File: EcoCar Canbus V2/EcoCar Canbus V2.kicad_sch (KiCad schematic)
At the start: 7 parts

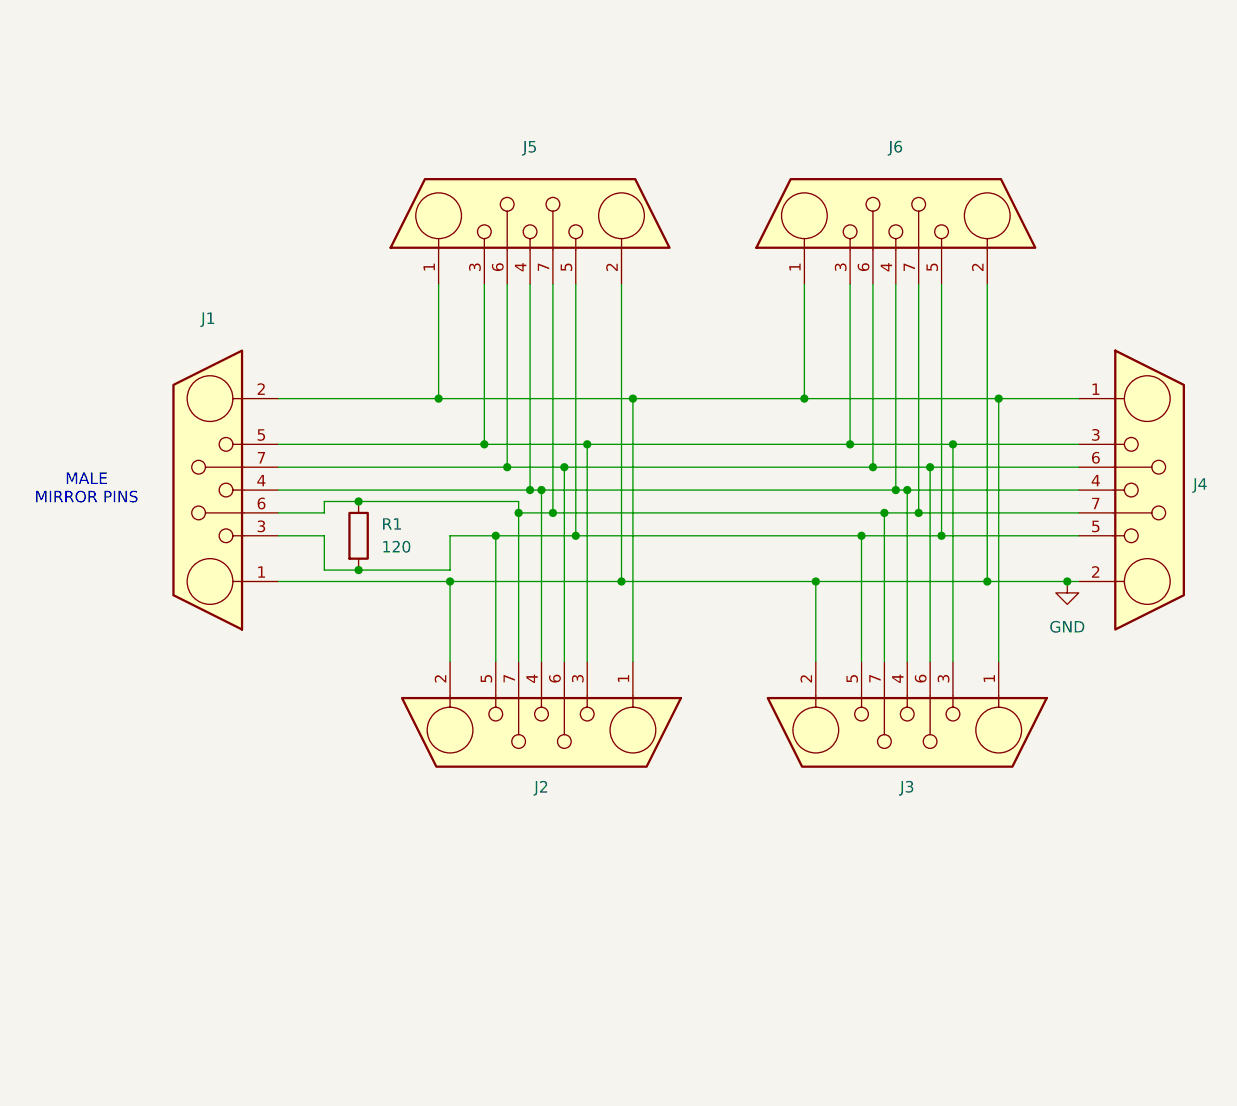
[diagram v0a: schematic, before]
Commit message: Changed connectors,footprints,pinouts. Almost ready :)
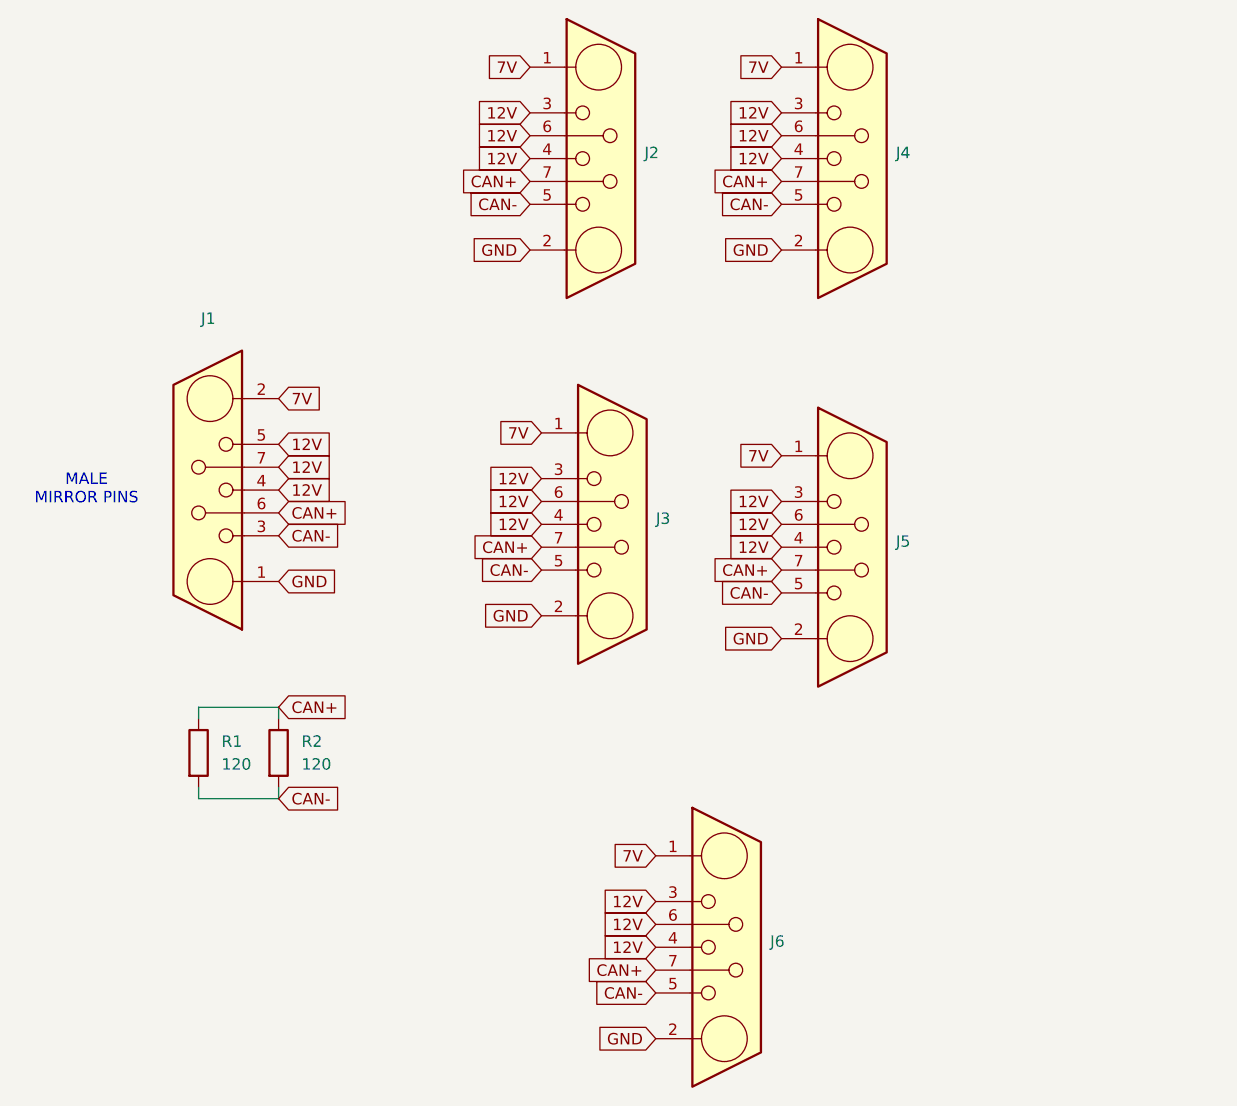
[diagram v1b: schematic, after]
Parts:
- added R2: 120, Resistor_THT:R_Axial_DIN0207_L6.3mm_D2.5mm_P7.62mm_Horizontal, symbol Device:R
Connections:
- net 7V: now reaches J1.2, J2.1, J3.1, J4.1, J5.1, J6.1
- net 12V: now reaches J1.5, J2.3, J3.3, J4.3, J5.3, J6.3
- net 12V: now also J1.4, J1.7, J2.4, J2.6, J3.4, J3.6, J4.4, J4.6, J5.4, J5.6, J6.4, J6.6
- net CAN-: now reaches J1.3, J2.5, J3.5, J4.5, J5.5, J6.5, R1.2
- net CAN-: now also R2.2
- net CAN+: now reaches J1.6, J2.7, J3.7, J4.7, J5.7, J6.7, R1.1
- net CAN+: now also R2.1
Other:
- moved on the sheet: J2, R1
